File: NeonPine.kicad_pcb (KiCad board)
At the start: 2 copper layers, 54.7 x 69 mm, 74 parts, among them J1 USB-C 6P (USB4125-GF-A), J2 SWD pogo pads, Q1 DMN15H310SE, Q11 MMBTA42, Q12 MMBTA42, Q13 MMBTA42, Q14 MMBTA42, Q15 MMBTA42, Q16 MMBTA42, Q17 MMBTA42, Q18 MMBTA42, Q19 MMBTA42, Q2 TEPT4400, Q20 MMBTA42, U1 CH32V003F4P6

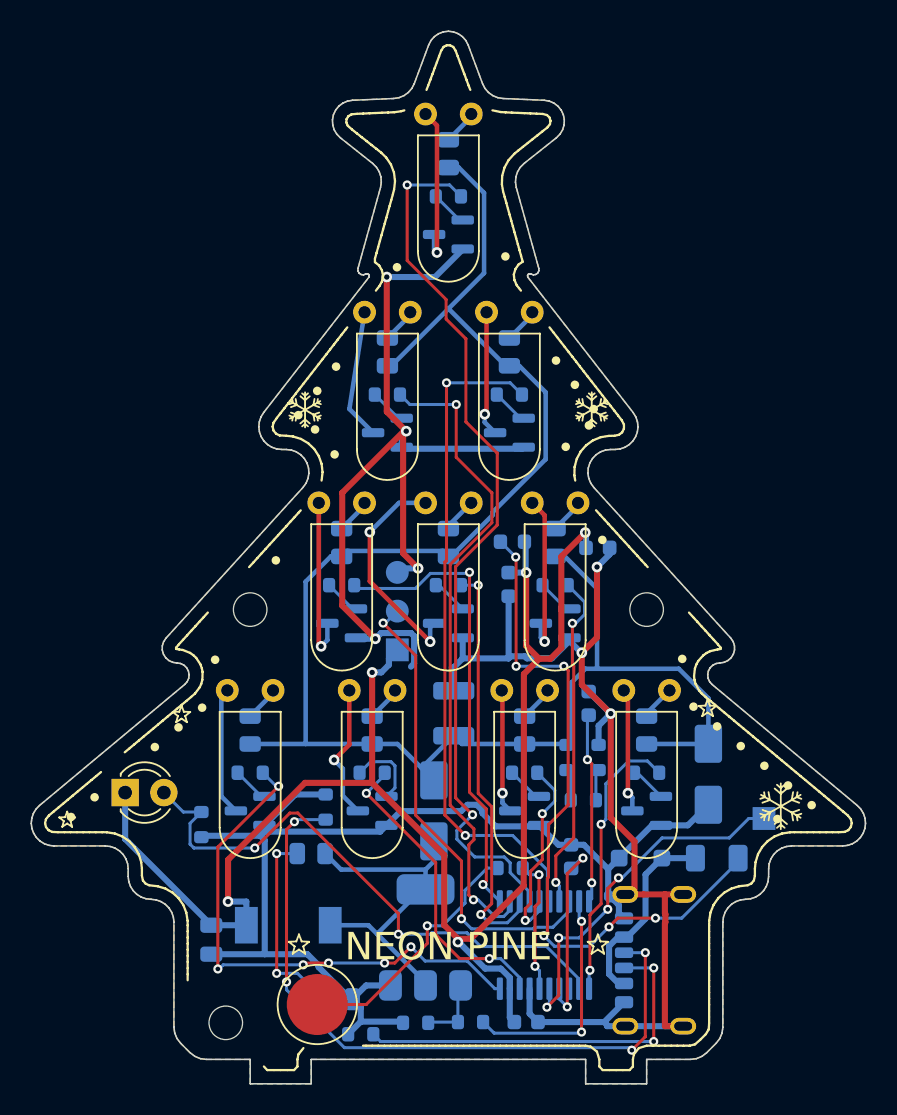
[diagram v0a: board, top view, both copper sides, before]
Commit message: incomplete big package ver
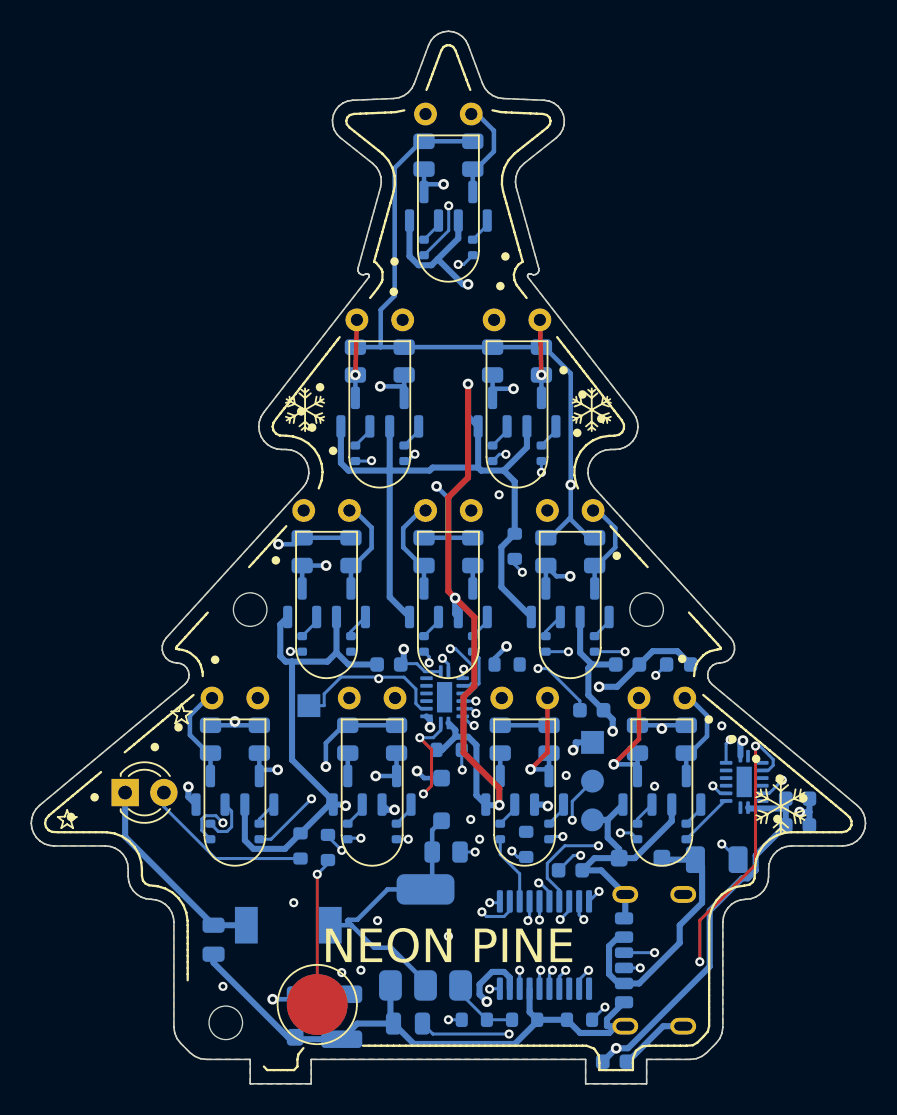
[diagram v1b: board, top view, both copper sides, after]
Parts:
- added C10: 100n, Capacitor_SMD:C_0603_1608Metric, B.Cu at (111.8, 84.1)
- added C9: 100n, Capacitor_SMD:C_0603_1608Metric, B.Cu at (96.1, 84.1)
- added Q21: MMBTA42, Package_TO_SOT_SMD:SOT-23, B.Cu at (101.6, 54.0)
- added Q22: MMBTA42, Package_TO_SOT_SMD:SOT-23, B.Cu at (97.1, 67.5)
- added Q23: MMBTA42, Package_TO_SOT_SMD:SOT-23, B.Cu at (106.1, 67.5)
- added Q24: MMBTA42, Package_TO_SOT_SMD:SOT-23, B.Cu at (93.6, 80.0)
- added Q25: MMBTA42, Package_TO_SOT_SMD:SOT-23, B.Cu at (101.6, 80.0)
- added Q26: MMBTA42, Package_TO_SOT_SMD:SOT-23, B.Cu at (109.6, 80.0)
- added Q27: MMBTA42, Package_TO_SOT_SMD:SOT-23, B.Cu at (87.6, 92.3)
- added Q28: MMBTA42, Package_TO_SOT_SMD:SOT-23, B.Cu at (96.6, 92.3)
- added Q29: MMBTA42, Package_TO_SOT_SMD:SOT-23, B.Cu at (106.6, 92.3)
- added Q30: MMBTA42, Package_TO_SOT_SMD:SOT-23, B.Cu at (115.6, 92.3)
- added R31: 150k, Resistor_SMD:R_0805_2012Metric, B.Cu at (98.4, 50.7)
- added R32: 150k, Resistor_SMD:R_0805_2012Metric, B.Cu at (93.9, 64.2)
- added R33: 150k, Resistor_SMD:R_0805_2012Metric, B.Cu at (102.9, 64.2)
- added R34: 150k, Resistor_SMD:R_0805_2012Metric, B.Cu at (90.4, 76.7)
- added R35: 150k, Resistor_SMD:R_0805_2012Metric, B.Cu at (98.4, 76.7)
- added R36: 150k, Resistor_SMD:R_0805_2012Metric, B.Cu at (106.4, 76.7)
- added R37: 150k, Resistor_SMD:R_0805_2012Metric, B.Cu at (84.4, 89.0)
- added R38: 150k, Resistor_SMD:R_0805_2012Metric, B.Cu at (93.4, 89.0)
- added R39: 150k, Resistor_SMD:R_0805_2012Metric, B.Cu at (103.4, 89.0)
- added R40: 150k, Resistor_SMD:R_0805_2012Metric, B.Cu at (112.4, 89.0)
- added R51: 22k, Resistor_SMD:R_0402_1005Metric, B.Cu at (101.6, 56.8)
- added R52: 22k, Resistor_SMD:R_0402_1005Metric, B.Cu at (97.1, 70.2)
- added R53: 22k, Resistor_SMD:R_0402_1005Metric, B.Cu at (106.1, 70.2)
- added R54: 22k, Resistor_SMD:R_0402_1005Metric, B.Cu at (93.6, 82.8)
- added R55: 22k, Resistor_SMD:R_0402_1005Metric, B.Cu at (101.6, 82.8)
- added R56: 22k, Resistor_SMD:R_0402_1005Metric, B.Cu at (109.6, 82.8)
- added R57: 22k, Resistor_SMD:R_0402_1005Metric, B.Cu at (87.6, 95.0)
- added R58: 22k, Resistor_SMD:R_0402_1005Metric, B.Cu at (96.6, 95.0)
- added R59: 22k, Resistor_SMD:R_0402_1005Metric, B.Cu at (106.6, 95.0)
- added R60: 22k, Resistor_SMD:R_0402_1005Metric, B.Cu at (115.6, 95.0)
- added U2: 74HC595BQ, Package_DFN_QFN:DHVQFN-16-1EP_2.5x3.5mm_P0.5mm_EP1x2mm, B.Cu at (99.8, 86.2)
- added U3: 74HC595BQ, Package_DFN_QFN:DHVQFN-16-1EP_2.5x3.5mm_P0.5mm_EP1x2mm, B.Cu at (119.4, 91.8)
- D1: value ES1D -> 200V 1A fast SOD-123F (verify P/N); footprint Diode_SMD:D_SMA -> Diode_SMD:D_SOD-123F
- D2: value SMAJ100A -> SMF100A; footprint Diode_SMD:D_SMA -> Diode_SMD:D_SOD-123F
- R41, R42, R43, R44, R45, R46, R47, R48, R49, R50: footprint Resistor_SMD:R_0603_1608Metric -> Resistor_SMD:R_0402_1005Metric
- TP3: value BUZZ/spare -> SR_CLK test
- moved D2 31.4 mm to (90.0, 107.2)
- moved TP3 30.8 mm to (90.8, 86.8), turned to -90 degrees
- moved C2 23.6 mm to (122.9, 92.9), turned to 0 degrees
- moved C1 22.4 mm to (122.9, 94.7)
- moved C4 21.2 mm to (93.0, 107.2), turned to -90 degrees
- moved J2 17.0 mm to (109.5, 91.8), turned to -90 degrees
- moved R7 14.9 mm to (104.3, 76.3)
- moved R4 14.4 mm to (108.6, 107.4)
- moved FB1 13.6 mm to (115.1, 84.1)
- moved R11 12.0 mm to (92.1, 96.1), turned to 90 degrees
- moved R3 8.93 mm to (100.0, 89.7), turned to 180 degrees
- moved R12 8.85 mm to (99.8, 96.4), turned to 0 degrees
- moved R5 7.24 mm to (103.8, 84.1), turned to 0 degrees
- moved R2 7.15 mm to (105.0, 107.4), turned to 0 degrees
- moved R9 6.65 mm to (90.3, 96.0), turned to 90 degrees
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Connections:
- net /B1 renamed Net-(Q11-B)
- net /B10 renamed Net-(Q20-B)
- net /B2 renamed Net-(Q12-B)
- net /B3 renamed Net-(Q13-B)
- net /B4 renamed Net-(Q14-B)
- net /B5 renamed Net-(Q15-B)
- net /B6 renamed Net-(Q16-B)
- net /B7 renamed Net-(Q17-B)
- net /B8 renamed Net-(Q18-B)
- net /B9 renamed Net-(Q19-B)
- net /BUZZ renamed /SR_CLK
- U1 pad 1: /LAMP10 -> /SR_LATCH
- U1 pad 12: /LAMP2 -> /LAMP5
- U1 pad 13: /LAMP5 -> /LAMP9
- U1 pad 14: /LAMP1 -> /LAMP2
- U1 pad 15: /LAMP9 -> /LAMP3
- U1 pad 16: /LAMP3 -> /LAMP6
- U1 pad 17: /LAMP6 -> /LAMP10
- U1 pad 3: unconnected-(U1-PD6-Pad3) -> /SR_DATA
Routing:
- net GND: track 208.0 -> 297.2 mm, vias 7 -> 11
- net /HV+: track 114.3 -> 176.8 mm, vias 0 -> 9
- net /SR_CLK: track 23.6 -> 68.0 mm
- net /SR_CHAIN: track 0.00 -> 31.9 mm, vias 0 -> 3
- net /LAMPA1: track 0.00 -> 30.1 mm, vias 0 -> 2
- net /VBUS_F: track 45.7 -> 16.8 mm, vias 6 -> 3
- net +5V: track 101.6 -> 129.1 mm, vias 5 -> 6
- net /LAMPA7: track 0.00 -> 24.0 mm, vias 0 -> 3
- net /LAMP1: track 58.4 -> 37.1 mm
- net /SWIO: track 31.2 -> 11.4 mm
- net /CC2: track 25.4 -> 5.78 mm
- net /LAMPA3: track 0.00 -> 19.2 mm, vias 0 -> 3
- net /CC1: track 45.8 -> 27.3 mm, vias 4 -> 3
- net /VFB: track 15.5 -> 33.8 mm, vias 2 -> 4
- net /LAMPA6: track 0.00 -> 16.7 mm, vias 0 -> 2
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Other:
- copper layers 2 -> 4
